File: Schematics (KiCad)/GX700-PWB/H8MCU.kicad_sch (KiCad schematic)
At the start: 11 parts

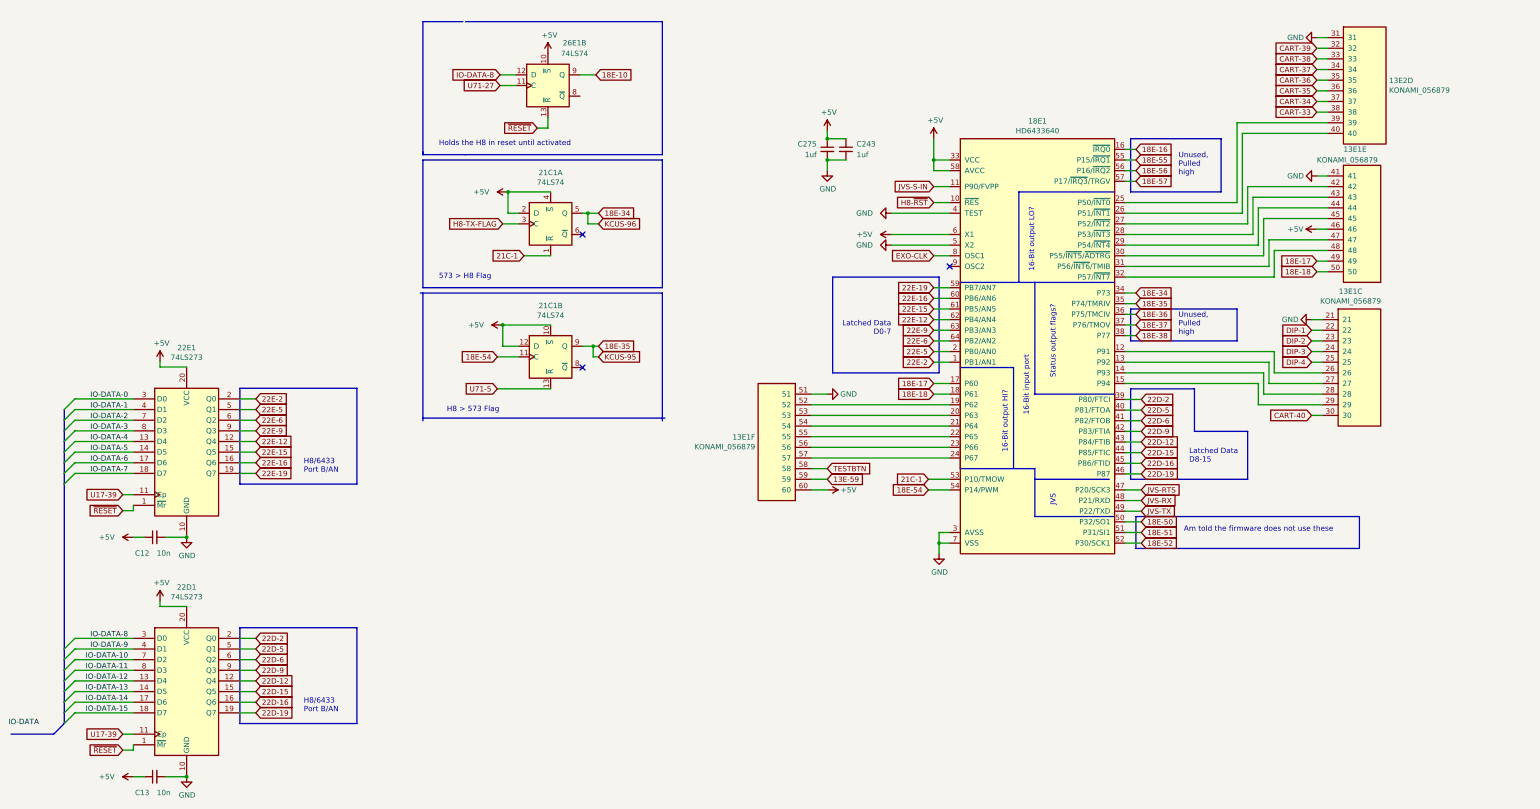
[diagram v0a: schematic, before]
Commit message: General Fixes
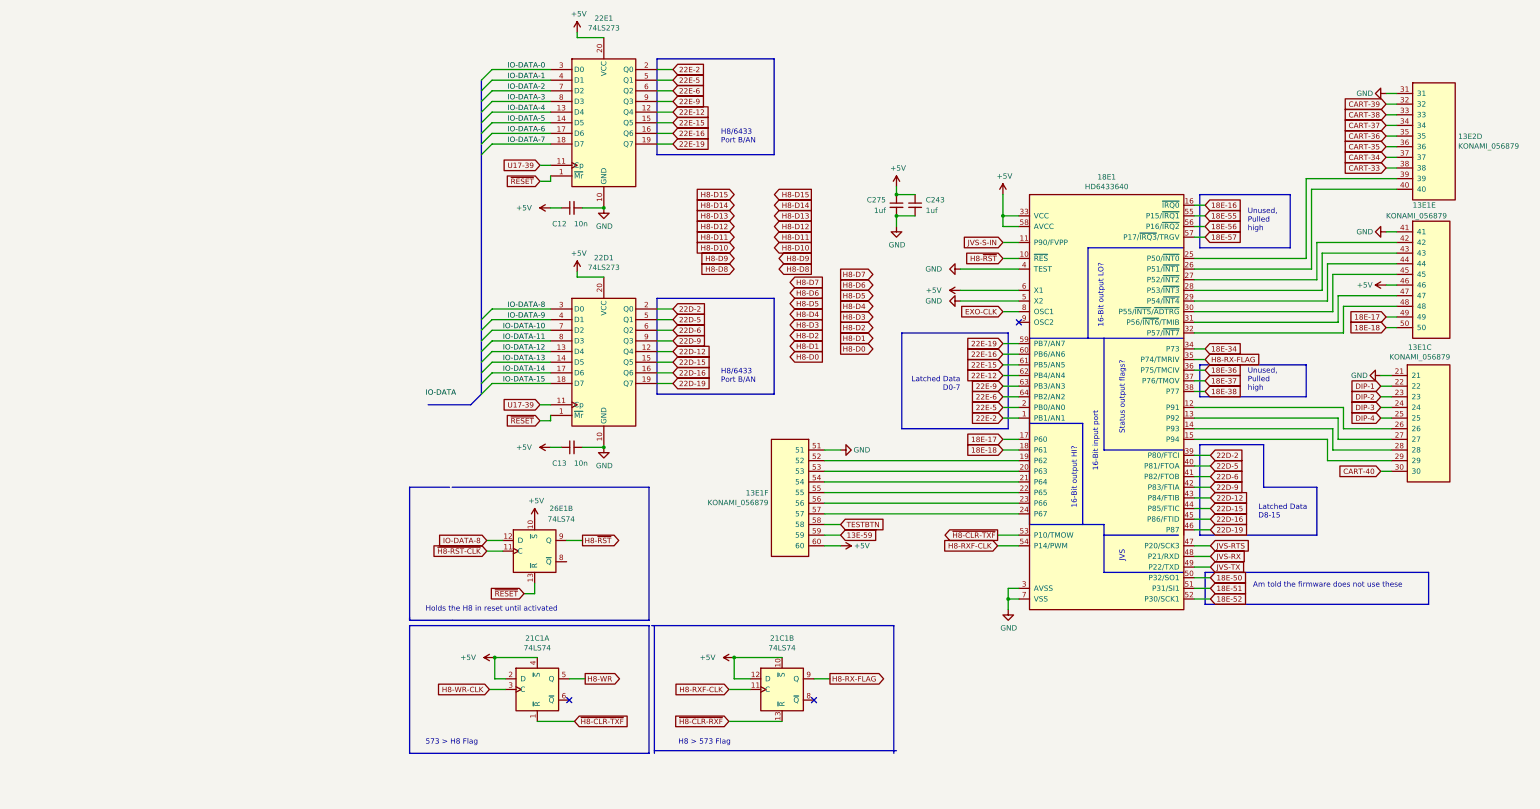
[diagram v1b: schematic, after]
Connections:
- net 18E-10 is gone; now on net H8-~{RST}: 26E1.9 (Q)
- net 18E-34: no longer 21C1.5 (Q)
- net 18E-35 renamed H8-RX-FLAG
- net 18E-54 renamed H8-RXF-CLK
- net 21C-1 renamed ~{H8-CLR-TXF}
- net H8-TX-FLAG renamed H8-WR-CLK
- net U71-27 renamed ~{H8-RST-CLK}
- net U71-5 renamed ~{H8-CLR-RXF}
- new net H8-WR: 21C1.5 (Q)
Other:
- moved on the sheet: 13E1C, 13E1E, 13E1F, 13E2D, 18E1, 21C1A, 21C1B, 22D1, 22E1, 26E1B, C12, C13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
